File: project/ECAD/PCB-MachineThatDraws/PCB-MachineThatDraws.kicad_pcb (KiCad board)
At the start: 2 copper layers, 53.5 x 83 mm, 29 parts, among them J1 SD_Card_Device, J10 Conn_02x03_Odd_Even, J11 Conn_02x03_Odd_Even, J2 SDA/SCL/VCC/GND, J3 Switch, J4 Limit_Switch_X, J5 Moteur, J6 Moteur, J7 Barrel_Jack_Switch, J8 Screw_Terminal_01x02, J9 Servo, U1 ESP32-S3-UNO, U2 R-78E5.0-1.0

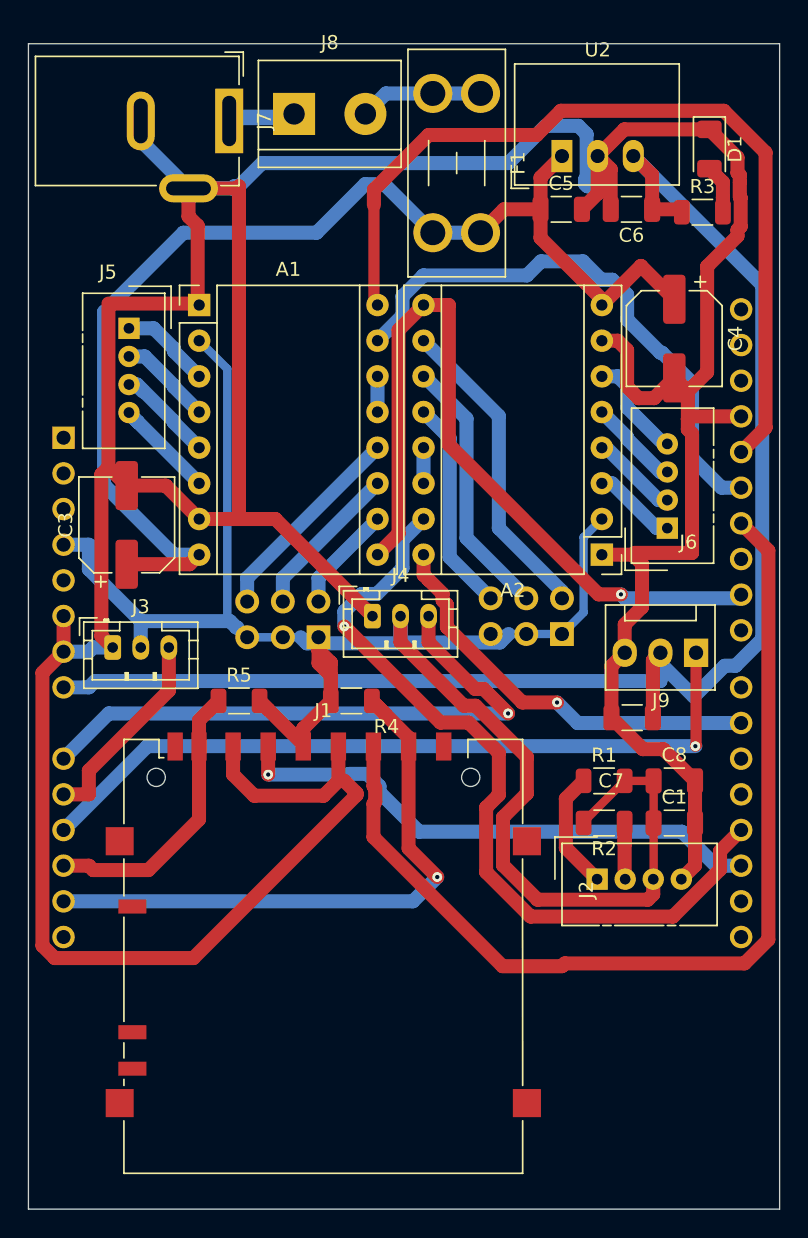
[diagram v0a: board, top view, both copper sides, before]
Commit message: up pcb
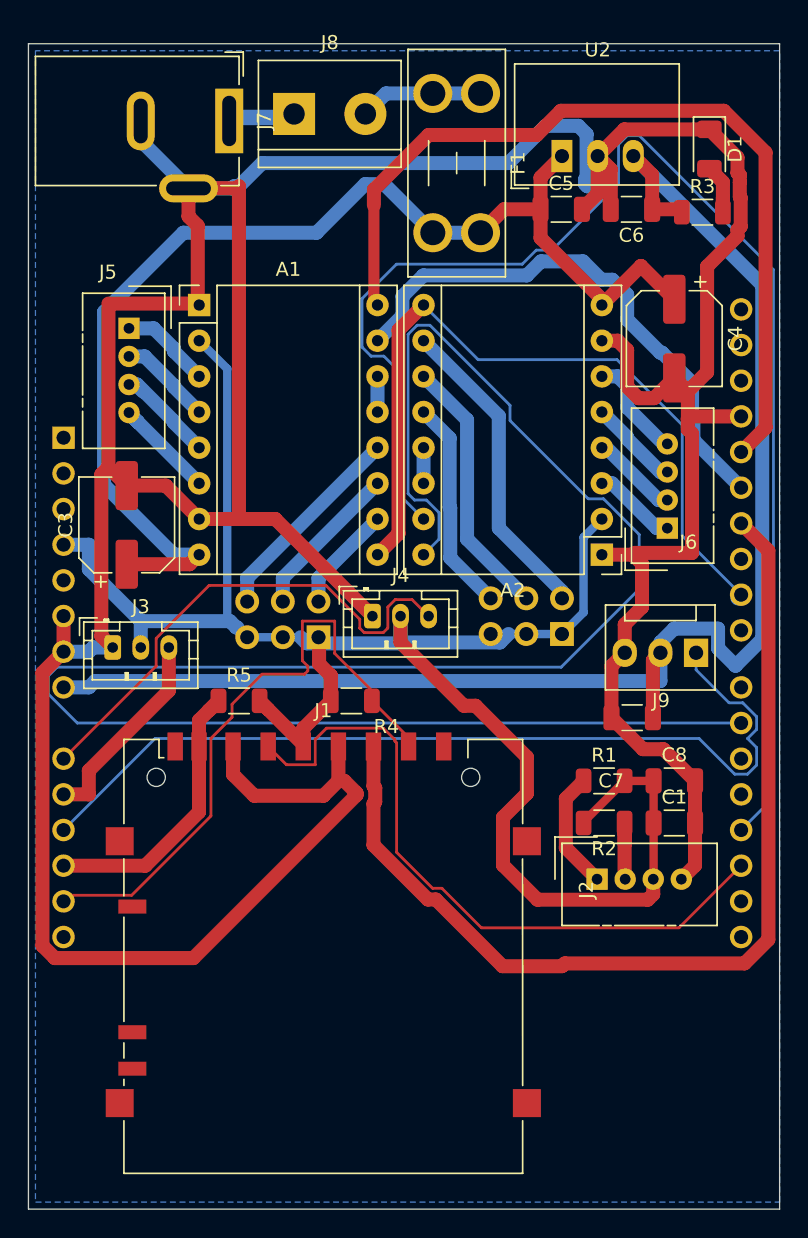
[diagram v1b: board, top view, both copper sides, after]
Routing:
- net D14: track 29.6 -> 141.1 mm, vias 1 -> 0
- net D10: track 57.0 -> 98.6 mm, vias 1 -> 0
- net D07: track 54.1 -> 64.3 mm, vias 1 -> 0
- net D18: track 38.7 -> 48.7 mm, vias 1 -> 0
- net D9: track 42.6 -> 36.4 mm, vias 1 -> 0
- net +3.3V: track 144.2 -> 142.0 mm
- net D05: track 43.8 -> 45.1 mm, vias 1 -> 0
- net Enable: track 56.3 -> 55.3 mm, vias 1 -> 0
- net D13: track 39.9 -> 39.1 mm
- net D19: track 21.3 -> 20.7 mm
- added copper zone on B.Cu, net GND

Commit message: maj pcb
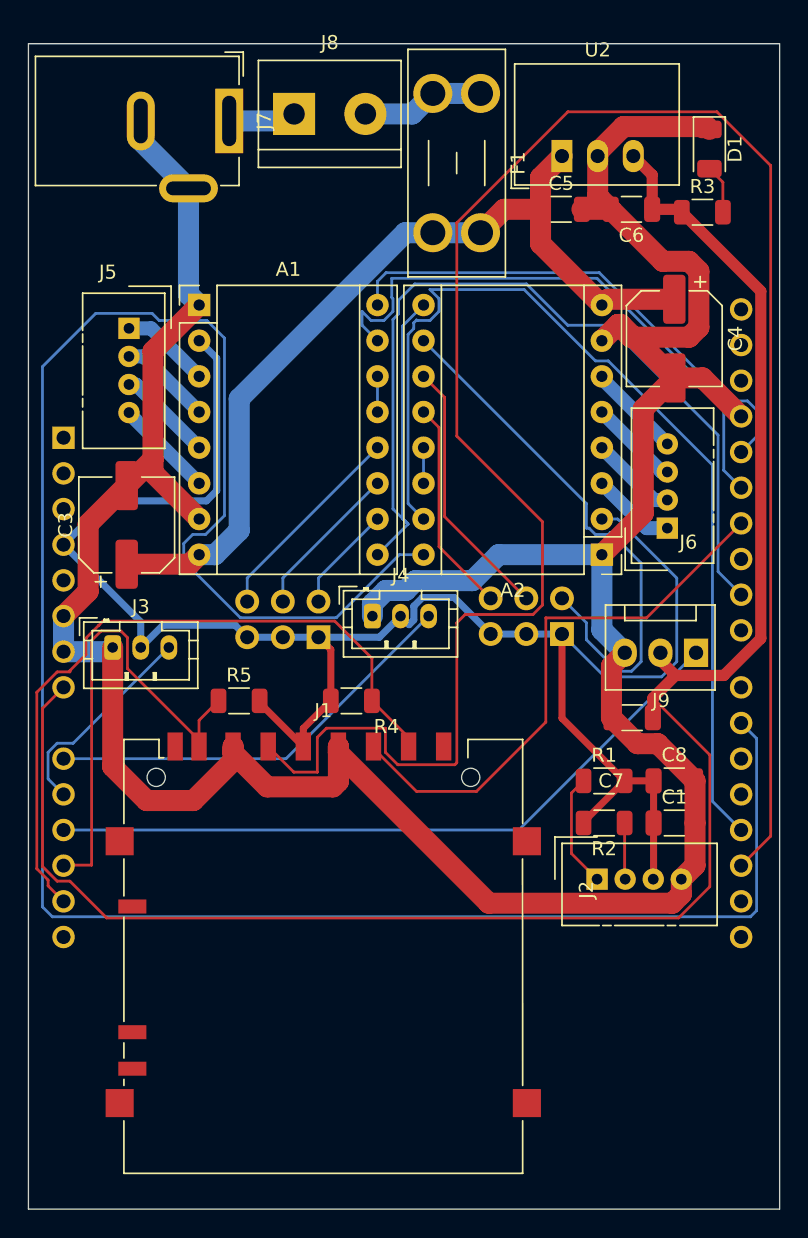
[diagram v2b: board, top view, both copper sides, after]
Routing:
- net D18: track 48.7 -> 143.4 mm
- net GND: track 302.4 -> 223.5 mm
- net D11: track 70.1 -> 39.8 mm
- net D10: track 98.6 -> 70.7 mm
- net D12: track 61.8 -> 36.4 mm
- net +5V: track 105.4 -> 130.6 mm
- net Enable: track 55.3 -> 75.8 mm
- net +12V: track 83.8 -> 63.8 mm
- net Net-(A2-MS1): track 22.4 -> 39.0 mm
- net D14: track 141.1 -> 157.1 mm
- net D19: track 20.7 -> 34.7 mm
- net D07: track 64.3 -> 50.3 mm
- net +3.3V: track 142.0 -> 129.6 mm
- net D9: track 36.4 -> 30.2 mm
- net D05: track 45.1 -> 50.8 mm
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- removed copper zone on B.Cu, net GND
